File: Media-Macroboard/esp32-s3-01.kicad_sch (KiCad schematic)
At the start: 25 parts, among them Q1 MMBT3904LT3G, Q2 MMBT3904LT3G, U1 ESP32-S3-WROOM-1, U2 USBLC6-2SC6, U3 CP2102N-Axx-xQFN20

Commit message: First productable version
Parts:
- C9: footprint Capacitor_SMD:C_0805_2012Metric_Pad1.18x1.45mm_HandSolder -> Capacitor_SMD:C_1206_3216Metric
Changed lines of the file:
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@@
 			)
 		)
-		(property "Footprint" "Capacitor_SMD:C_0805_2012Metric_Pad1.18x1.45mm_HandSolder"
+		(property "Footprint" "Capacitor_SMD:C_1206_3216Metric"
 			(at 69.85 32.7152 0)
 			(effects

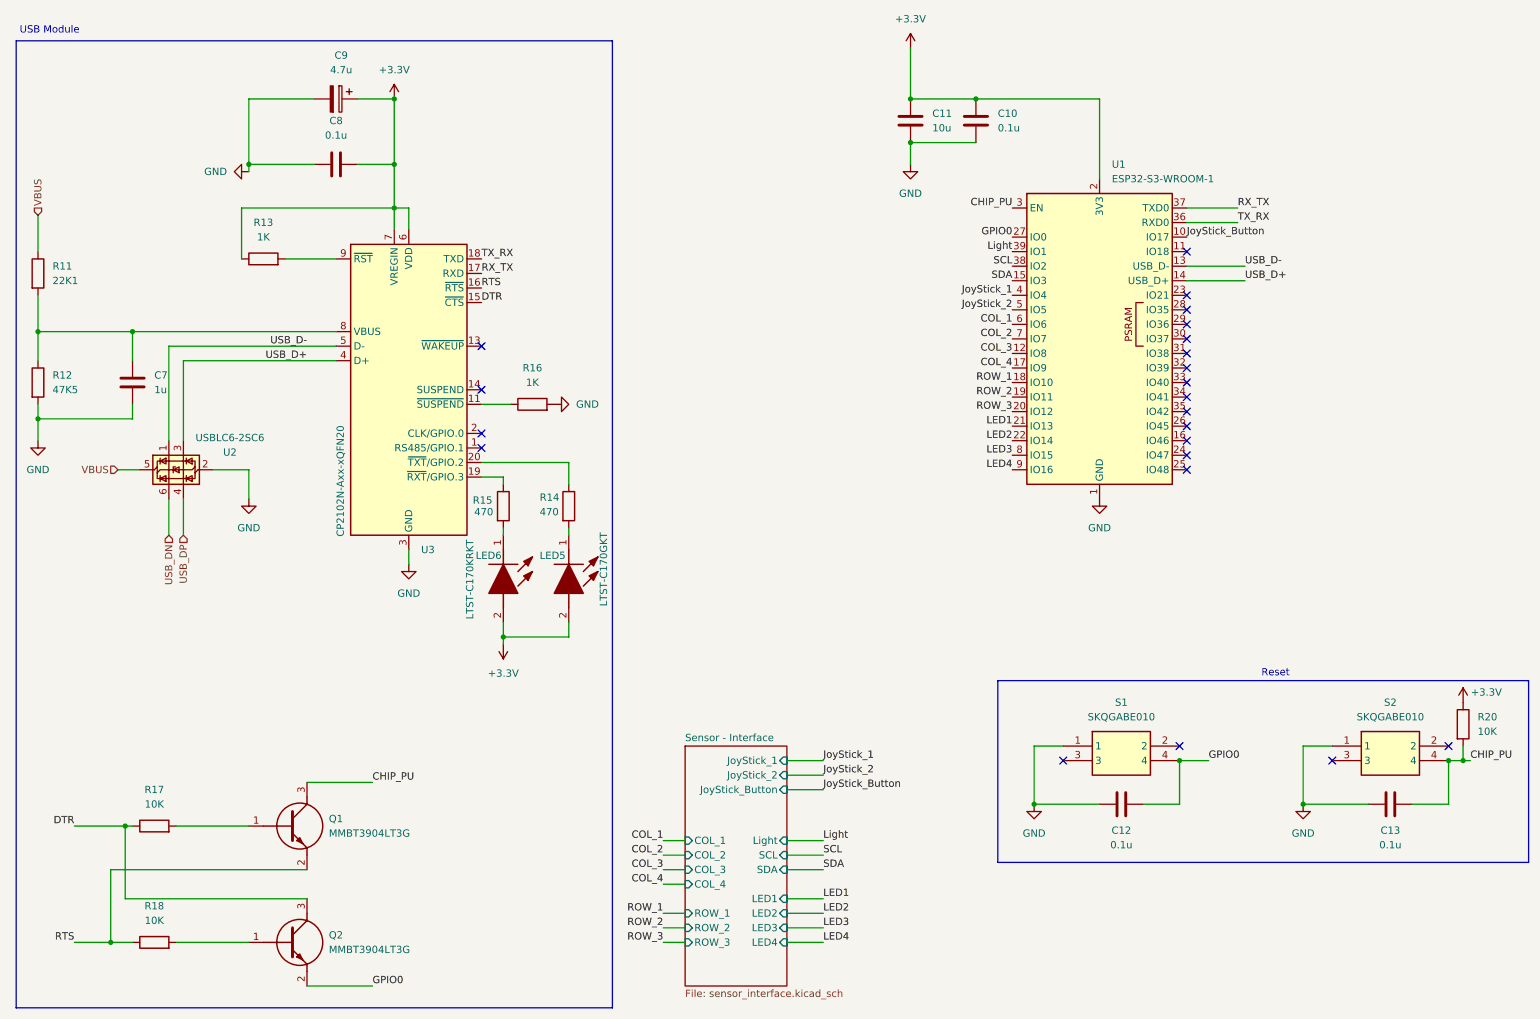
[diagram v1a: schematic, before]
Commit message: Update
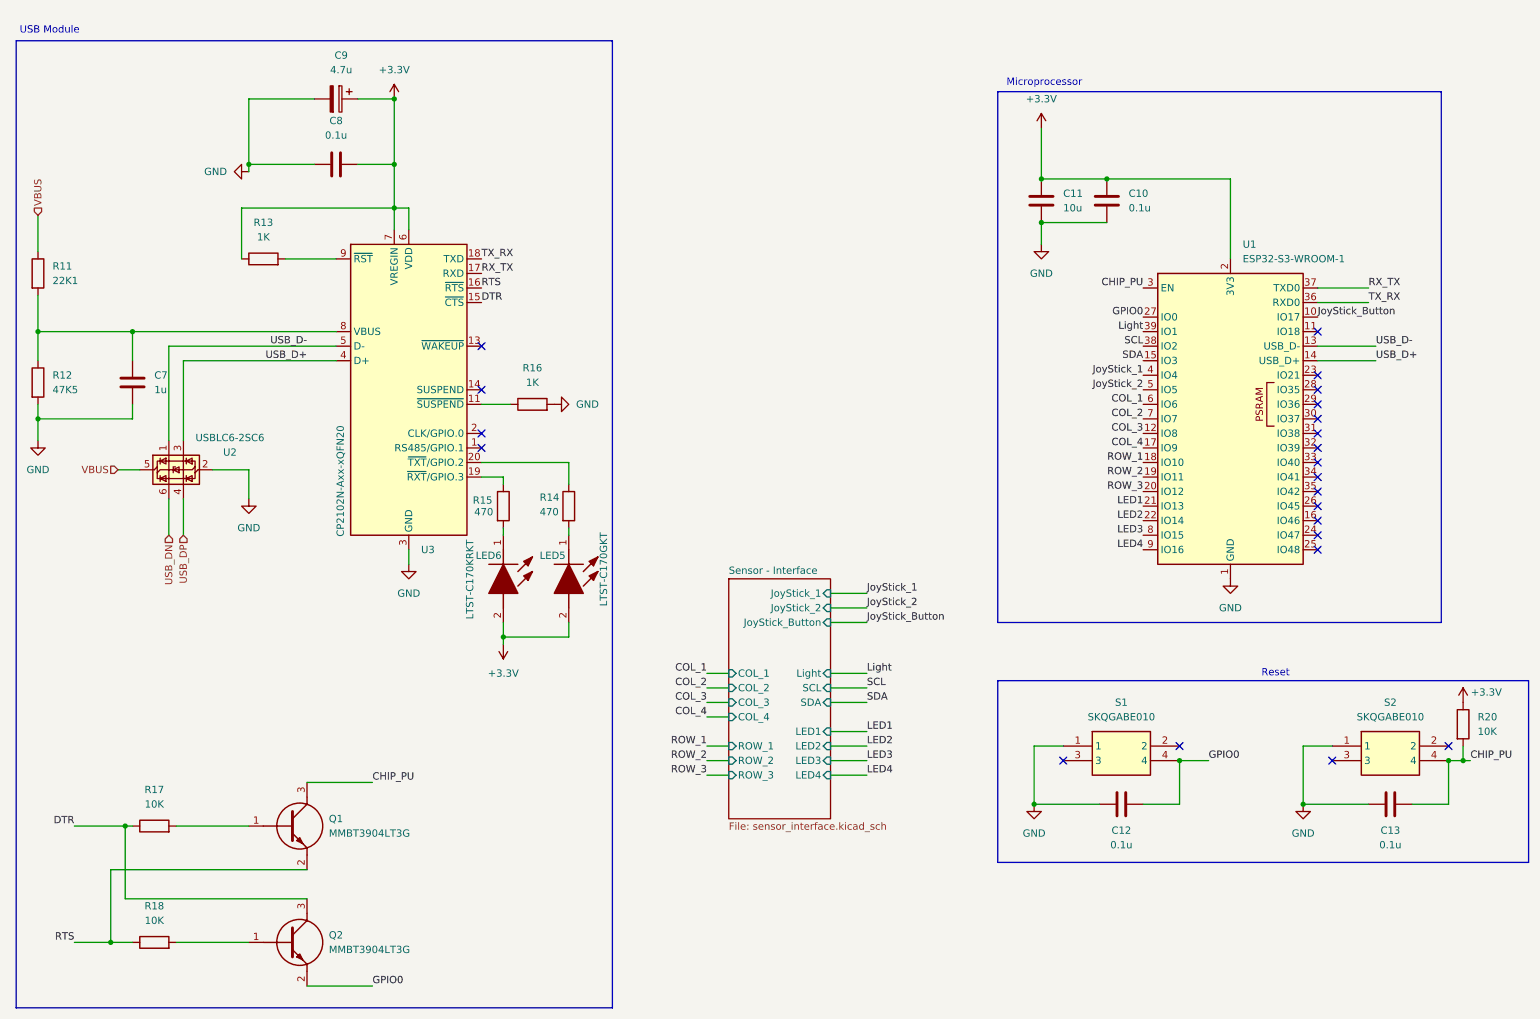
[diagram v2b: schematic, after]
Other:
- note added: "Microprocessor"
- moved on the sheet: C10, C11, U1
